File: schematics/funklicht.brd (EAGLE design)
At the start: 50 x 50.1 mm, 23 parts, among them IC2 5V, SW1 push, SW2 push, SW3 push, SW4 push

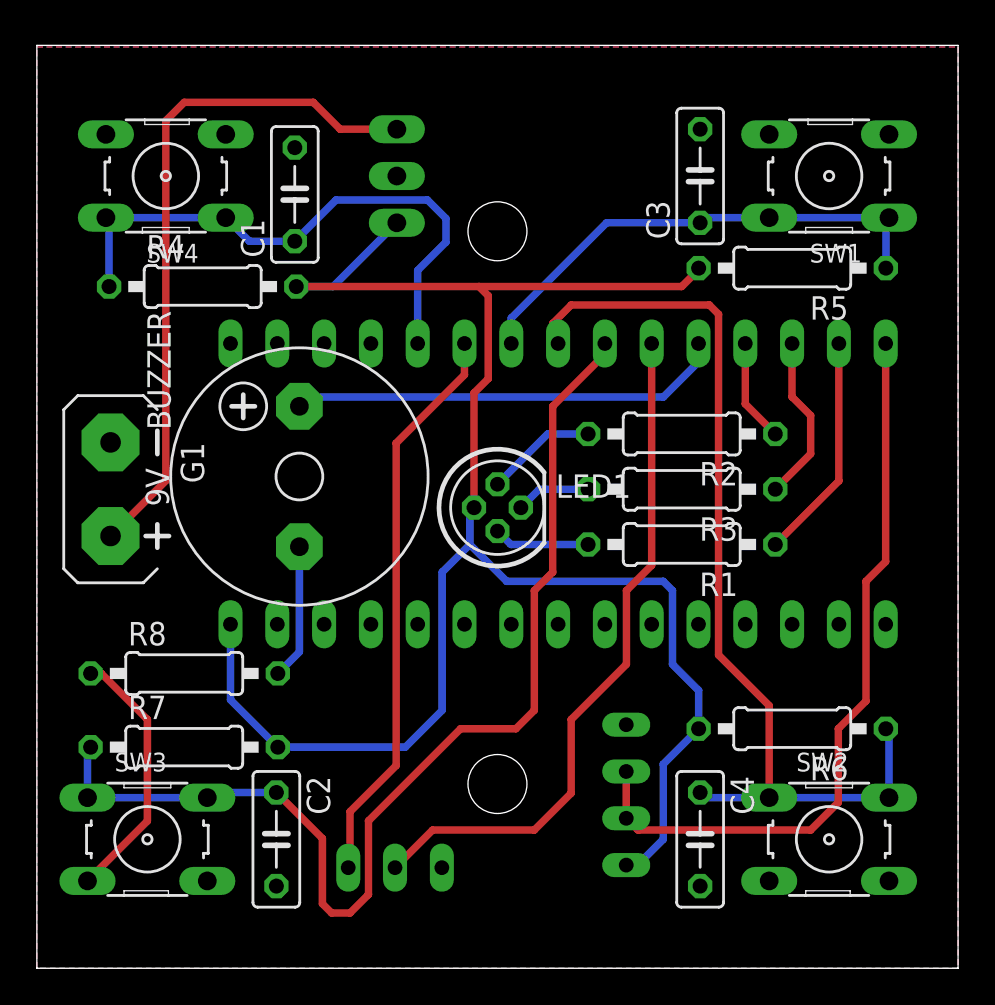
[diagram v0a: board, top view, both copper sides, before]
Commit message: schematics done
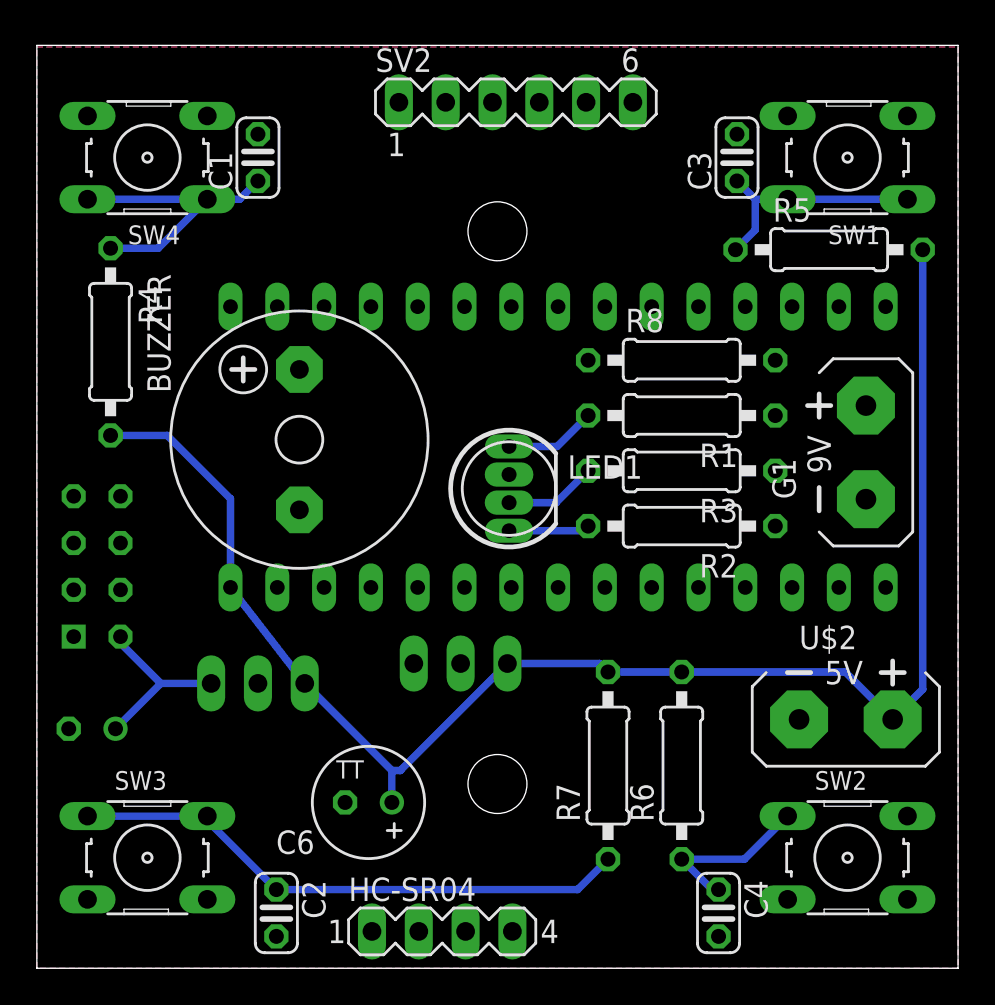
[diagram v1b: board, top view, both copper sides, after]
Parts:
- removed U$3: TRANSMITTER, funkmodule:TRANSMITTER
- added 3.3V: LM3940, voltage_regulator:78XXS
- added C5, C6: 100uF, rcl:TT2D6
- added HC-SR04: (no value), con-lstb:MA04-1
- added SV2: (no value), con-lstb:MA06-1
- added U$4: NRF24L01, funkmodule:NRF24L01
- C1, C2, C3, C4: device rcl:C050-025X075 -> rcl:C025-024X044
- LED1: value RGB -> (none)
- U$2: value RECIEVER -> AB5V; device funkmodule:RECIEVER -> power_supply:AB9V
- moved G1 41.0 mm to (45.0, 28.0), turned to 0 degrees
- moved R8 31.9 mm to (35.0, 33.0)
- moved U$2 30.0 mm to (43.9, 13.5), flipped to the top, turned to 270 degrees
- moved IC2 29.6 mm to (23.0, 14.0), turned to 180 degrees
- moved R7 23.0 mm to (31.0, 11.0), turned to 90 degrees
- moved R1 7.00 mm to (35.0, 30.0)
- moved R6 6.32 mm to (35.0, 11.0), turned to 90 degrees
- moved R4 5.83 mm to (4.00, 34.0), turned to 270 degrees
- moved R2 5.00 mm to (35.0, 24.0)
- moved C4 4.12 mm to (37.0, 3.00)
- moved C2 4.00 mm to (13.0, 3.00)
- moved C1 2.83 mm to (12.0, 44.0)
- moved C3 2.24 mm to (38.0, 44.0)
- moved R5 2.24 mm to (43.0, 39.0), turned to 0 degrees
- moved BUZZER 2.00 mm to (14.2, 28.7)
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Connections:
- removed net TX_ENABLE: U$1.D7, U$3.TX_ENABLE
- removed net VDD: IC2.OUT, LED1.VCC, R4.2, R5.2, R6.2, R7.2, U$1.VIN, U$2.VCC
- new net N$10: U$1.D8, U$4.CE
- new net N$11: R3.1, SV2.4, U$1.D5
- new net N$12: R1.1, SV2.3, U$1.D3
- new net N$13: HC-SR04.3, U$1.D2
- new net N$14: HC-SR04.2, U$1.D4
- new net N$21: SV2.1, U$1.D7
- new net N$22: SV2.2, U$1.A5
- new net N$8: U$1.D11, U$4.MOSI
- new net N$9: U$1.D10, U$4.CSN
- new net VCC: 3.3V.IN, C6.+, HC-SR04.1, IC2.OUT, R4.2, R5.2, R6.2, R7.2, U$1.VIN, U$2.+
- net GND: now also 3.3V.GND, C5.-, C6.-, HC-SR04.4, LED1.GND, SV2.6, U$2.-, U$4.GND; no longer U$2.GND, U$3.GND
- net N$1: now also U$1.A0; no longer U$1.D2
- net N$15: now also U$1.A1; no longer U$1.D4
- net N$16: now also U$1.A2; no longer U$1.D5
- net N$17: now also U$1.A3; no longer U$1.D6
- net N$18: no longer U$1.D8
- net N$2: now also R2.1, SV2.5, U$1.D6; no longer U$1.D3, U$3.DATA
- net N$3: now also U$4.MISO; no longer U$2.DATA, U$2.DATA1
- net N$4: now also 3.3V.OUT, C5.+, U$4.VCC; no longer R1.1, U$1.D11
- net N$5: now also U$1.D9, U$4.IRQ; no longer R3.1, U$1.D10
- net N$6: now also U$1.D13, U$4.SCK; no longer R2.1, U$1.D9
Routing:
- net VDD: track 100.4 -> 0.00 mm
- net VCC: track 0.00 -> 84.8 mm
- net N$16: track 52.4 -> 9.40 mm
- net N$3: track 40.9 -> 0.00 mm
- net TX_ENABLE: track 37.5 -> 0.00 mm
- net N$20: track 37.3 -> 0.00 mm
- net N$2: track 31.1 -> 0.00 mm
- net N$17: track 60.4 -> 30.7 mm
- net N$18: track 23.7 -> 0.00 mm
- net N$1: track 31.6 -> 16.0 mm
- net GND: track 14.3 -> 0.00 mm
- net N$15: track 26.9 -> 12.9 mm
- net N$5: track 9.12 -> 0.00 mm
- net N$19: track 7.36 -> 0.00 mm
- net N$6: track 5.59 -> 0.00 mm
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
